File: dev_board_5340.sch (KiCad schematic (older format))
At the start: 41 parts, among them J1 Conn_01x04_Male, J2 USB_C_Receptacle_USB2.0, U1 nrf5340, U2 USBLC6-2SC6, U3 W25Q128JVS, Y1 Crystal_GND2_Small

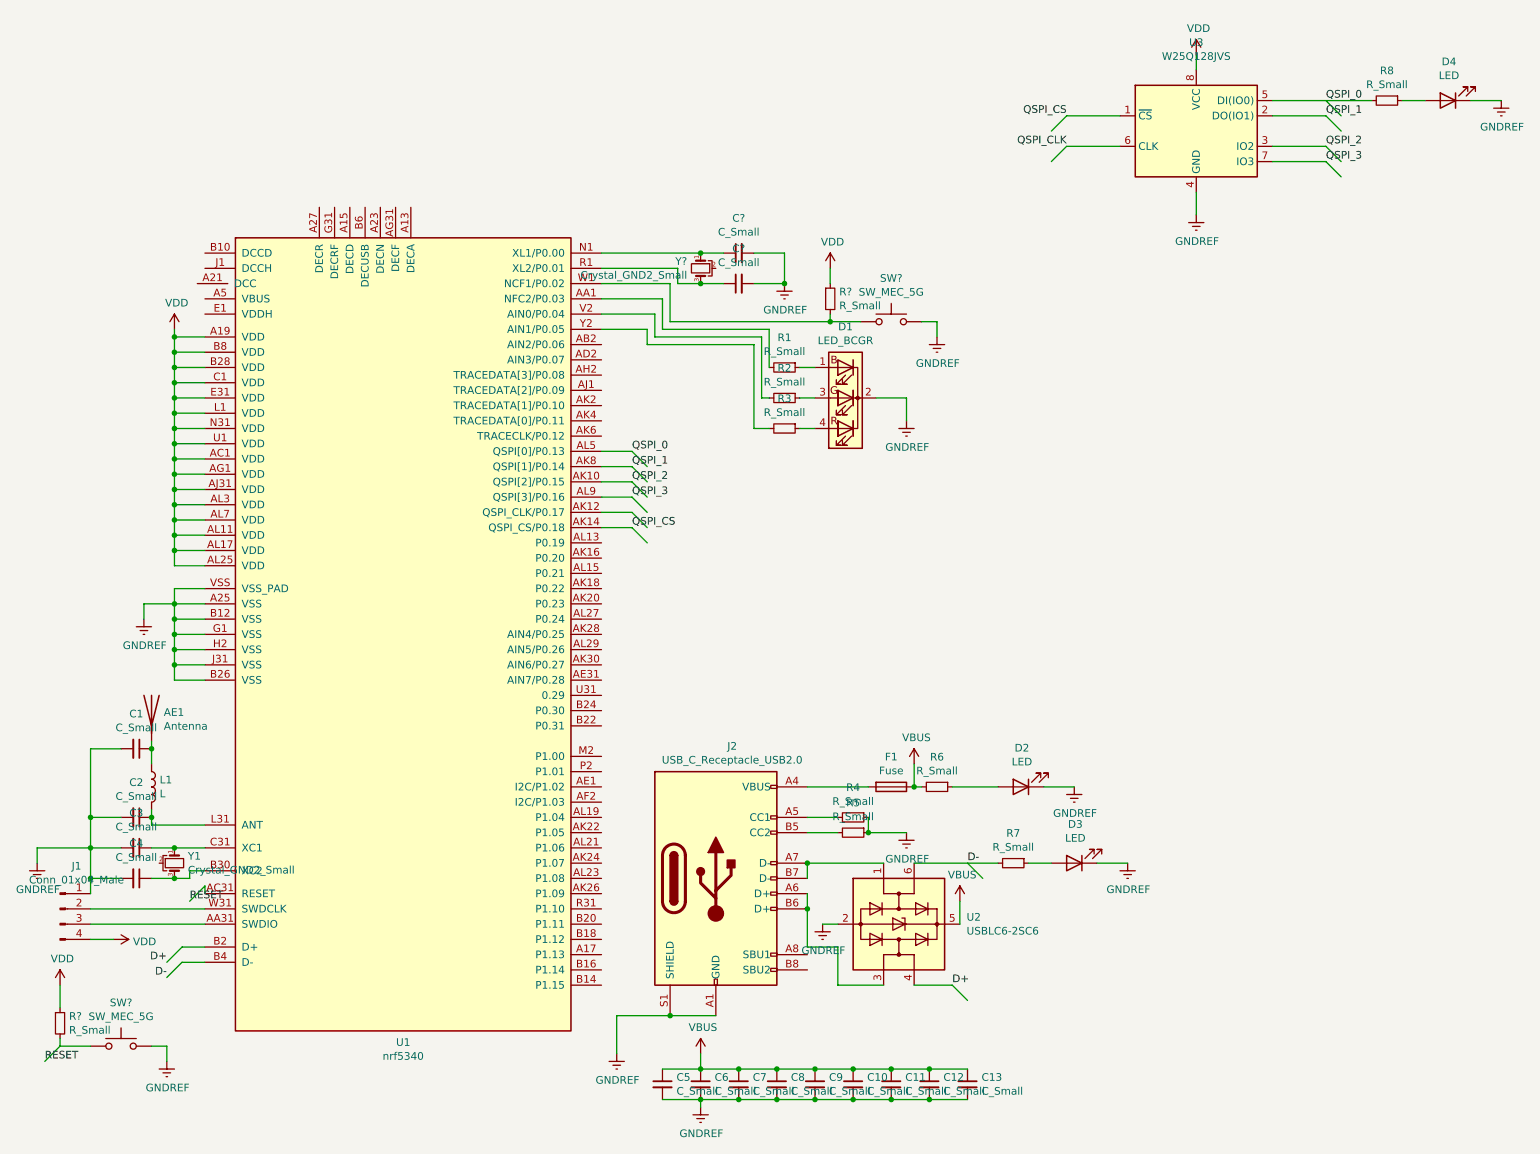
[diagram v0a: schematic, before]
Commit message: change schematic
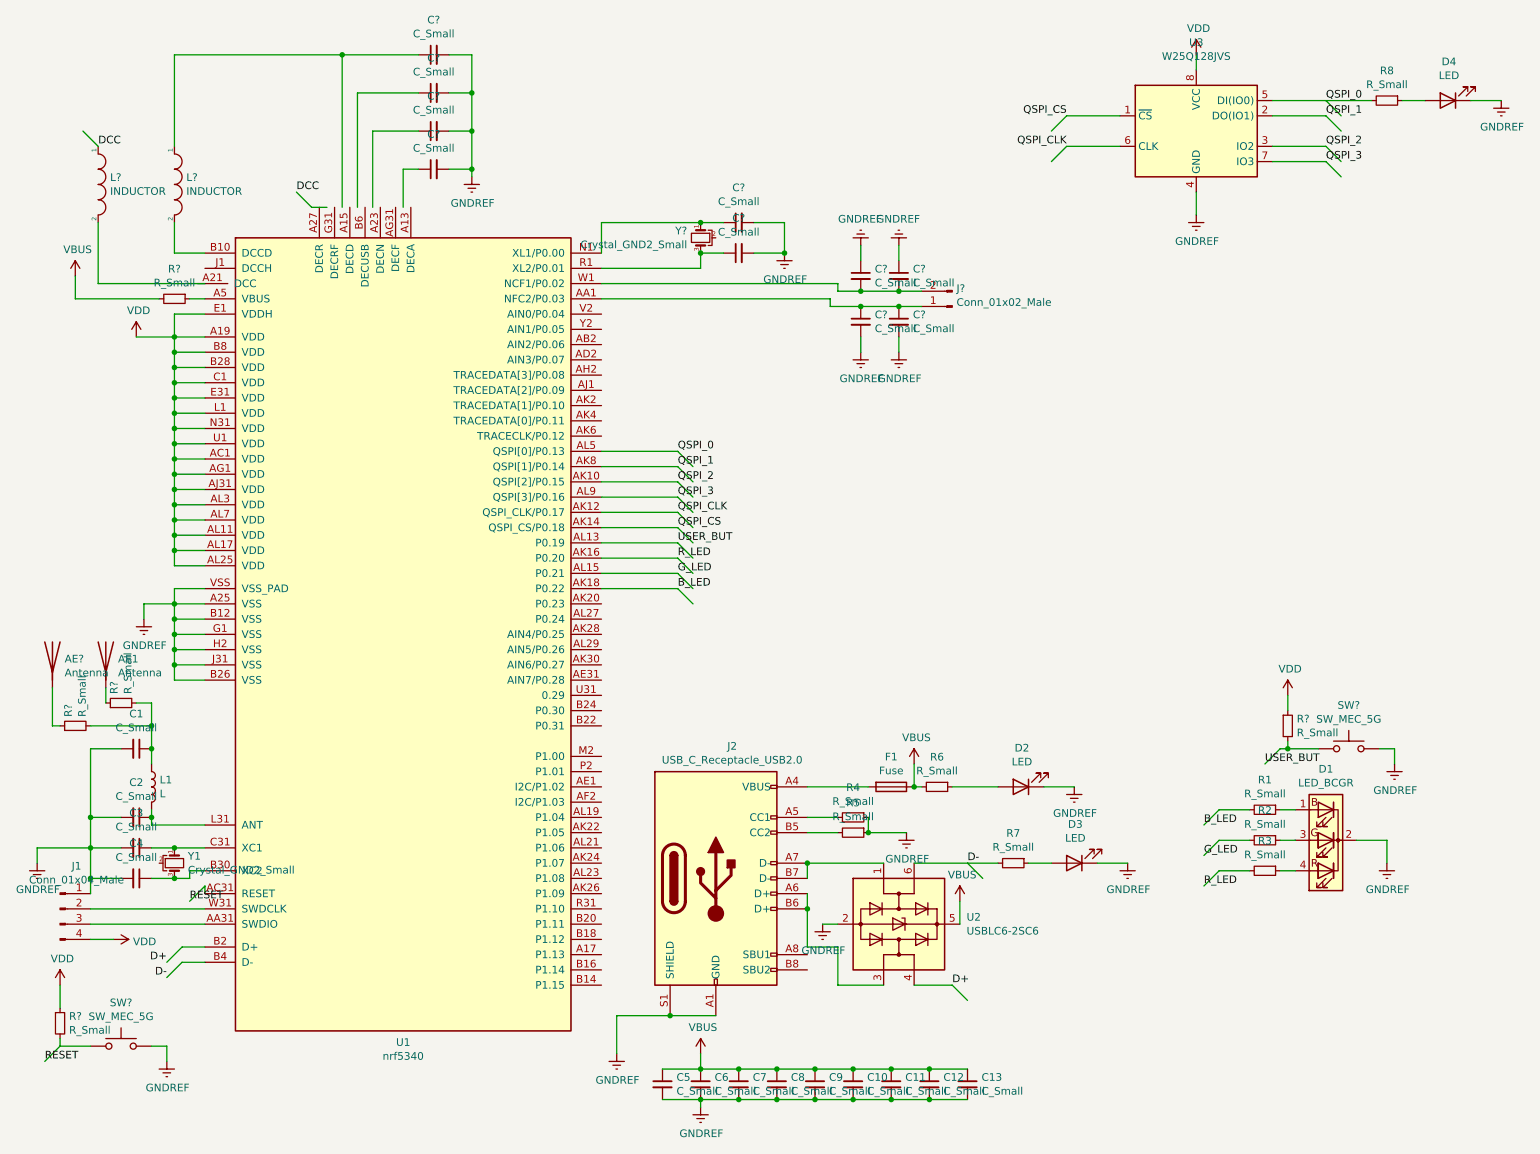
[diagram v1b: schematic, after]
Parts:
- added AE?: Antenna, symbol Device:Antenna
- added C? (x8): C_Small, symbol Device:C_Small
- added J?: Conn_01x02_Male, symbol Connector:Conn_01x02_Male
- added L? (x2): INDUCTOR, symbol pspice:INDUCTOR
- added R? (x3): R_Small, symbol Device:R_Small
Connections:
- net labels added: B_LED, DCC, G_LED, R_LED, USER_BUT
- wire segments 174 -> 213
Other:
- moved on the sheet: AE1, C?, D1, R1, R2, R3, R?, SW?, Y?
